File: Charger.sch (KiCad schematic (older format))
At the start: 2 parts

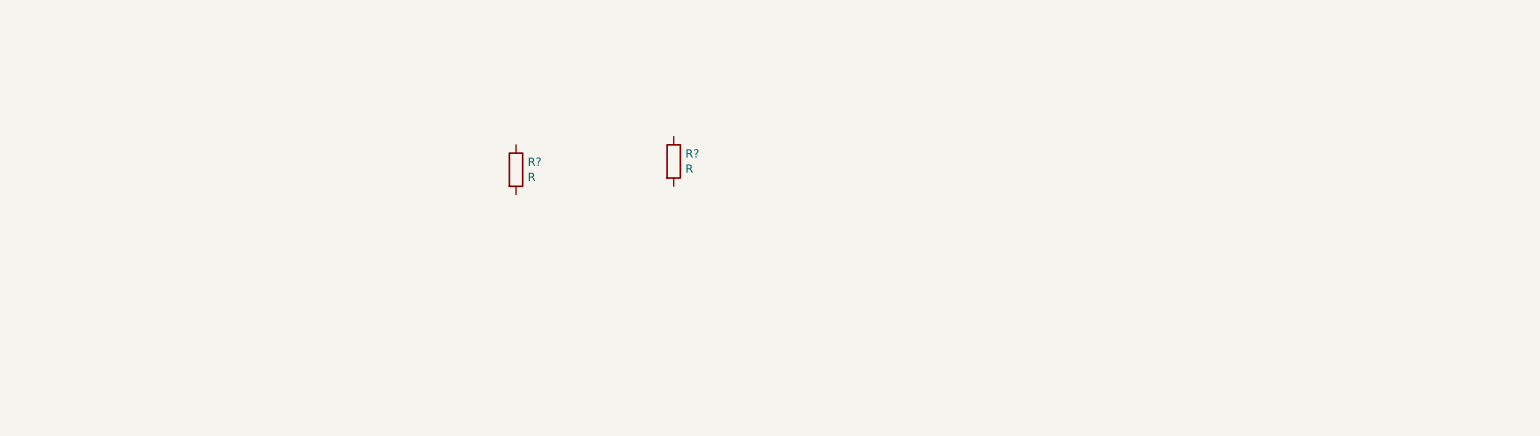
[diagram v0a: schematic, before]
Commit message: added ckt
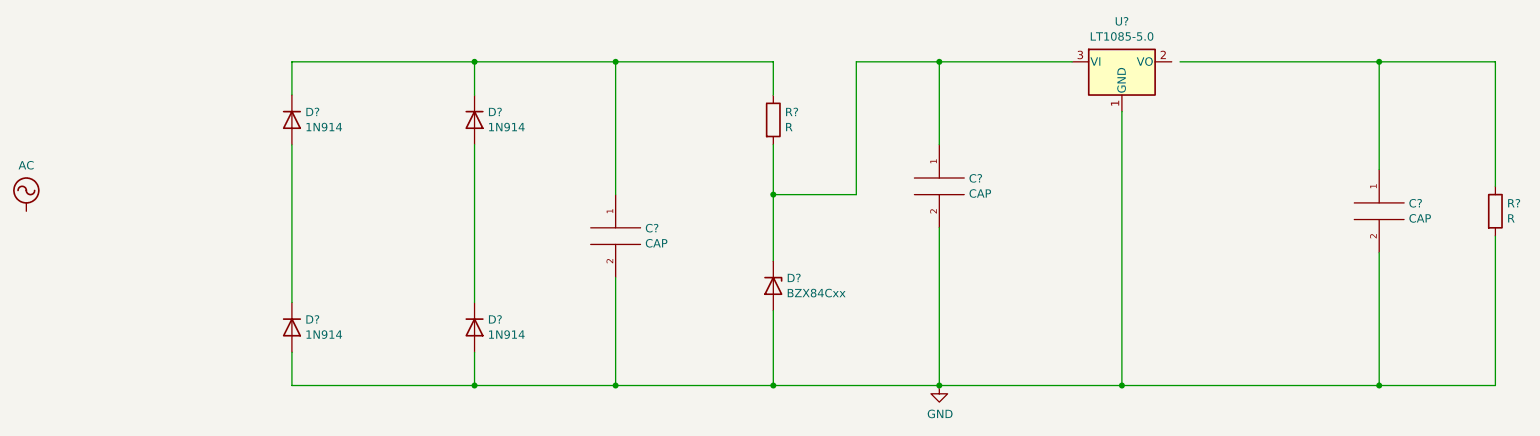
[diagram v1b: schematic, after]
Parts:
- removed R? (x2): R, symbol Device:R
- added C? (x3): CAP, symbol pspice:CAP
- added D? (x4): 1N914, Diode_THT:D_DO-35_SOD27_P7.62mm_Horizontal, symbol Diode:1N914
- added D?: BZX84Cxx, Diode_SMD:D_SOT-23_ANK, symbol Diode:BZX84Cxx
- added R? (x2): R, symbol Device:R
- added U?: LT1085-5.0, symbol Regulator_Linear:LT1085-5.0
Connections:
- net labels added: AC, GND
- wire segments 0 -> 35
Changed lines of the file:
@@
 $EndDescr
 $Comp
+L Diode:1N914 D?
+U 1 1 6031057C
+P 3100 2550
+F 0 "D?" V 3054 2630 50  0000 L CNN
+F 1 "1N914" V 3145 2630 50  0000 L CNN
+F 2 "Diode_THT:D_DO-35_SOD27_P7.62mm_Horizontal" H 3100 2375 50  0001 C CNN
+F 3 "http://www.vishay.com/docs/85622/1n914.pdf" H 3100 2550 50  0001 C CNN
+	1    3100 2550
+	0    1    1    0
+$EndComp
+$Comp
+L Diode:1N914 D?
+U 1 1 60311C82
+P 3100 3800
+F 0 "D?" V 3054 3880 50  0000 L CNN
+F 1 "1N914" V 3145 3880 50  0000 L CNN
+F 2 "Diode_THT:D_DO-35_SOD27_P7.62mm_Horizontal" H 3100 3625 50  0001 C CNN
+F 3 "http://www.vishay.com/docs/85622/1n914.pdf" H 3100 3800 50  0001 C CNN
+	1    3100 3800
+	0    1    1    0
+$EndComp
+$Comp
+L Diode:1N914 D?
+U 1 1 60312AAD
+P 4200 2550
+F 0 "D?" V 4154 2630 50  0000 L CNN
+F 1 "1N914" V 4245 2630 50  0000 L CNN
+F 2 "Diode_THT:D_DO-35_SOD27_P7.62mm_Horizontal" H 4200 2375 50  0001 C CNN
+F 3 "http://www.vishay.com/docs/85622/1n914.pdf" H 4200 2550 50  0001 C CNN
+	1    4200 2550
+	0    1    1    0
+$EndComp
+$Comp
+L Diode:1N914 D?
+U 1 1 60313CDB
+P 4200 3800
+F 0 "D?" V 4154 3880 50  0000 L CNN
+F 1 "1N914" V 4245 3880 50  0000 L CNN
+F 2 "Diode_THT:D_DO-35_SOD27_P7.62mm_Horizontal" H 4200 3625 50  0001 C CNN
+F 3 "http://www.vishay.com/docs/85622/1n914.pdf" H 4200 3800 50  0001 C CNN
+	1    4200 3800
+	0    1    1    0
+$EndComp
+$Comp
+L pspice:CAP C?
+U 1 1 60316869
+P 5050 3250
+F 0 "C?" H 5228 3296 50  0000 L CNN
+F 1 "CAP" H 5228 3205 50  0000 L CNN
+F 2 "" H 5050 3250 50  0001 C CNN
+F 3 "~" H 5050 3250 50  0001 C CNN
+	1    5050 3250
+	1    0    0    -1
+$EndComp
+$Comp
+L Diode:BZX84Cxx D?
+U 1 1 603170B0
+P 6000 3550
+F 0 "D?" V 5954 3630 50  0000 L CNN
+F 1 "BZX84Cxx" V 6045 3630 50  0000 L CNN
+F 2 "Diode_SMD:D_SOT-23_ANK" H 6000 3375 50  0001 C CNN
+F 3 "https://diotec.com/tl_files/diotec/files/pdf/datasheets/bzx84c2v4.pdf" H 6000 3550 50  0001 C CNN
+	1    6000 3550
+	0    1    1    0
+$EndComp
+$Comp
 L Device:R R?
-U 1 1 60309E92
-P 5400 2800
-F 0 "R?" H 5470 2846 50  0000 L CNN
-F 1 "R" H 5470 2755 50  0000 L CNN
-F 2 "" V 5330 2800 50  0001 C CNN
-F 3 "~" H 5400 2800 50  0001 C CNN
-	1    5400 2800
+U 1 1 60317AB7
+P 6000 2550
+F 0 "R?" H 6070 2596 50  0000 L CNN
+F 1 "R" H 6070 2505 50  0000 L CNN
+F 2 "" V 5930 2550 50  0001 C CNN
+F 3 "~" H 6000 2550 50  0001 C CNN
+	1    6000 2550
+	1    0    0    -1
+$EndComp
+$Comp
+L pspice:CAP C?
+U 1 1 60318512
+P 7000 2950
+F 0 "C?" H 7178 2996 50  0000 L CNN
+F 1 "CAP" H 7178 2905 50  0000 L CNN
+F 2 "" H 7000 2950 50  0001 C CNN
+F 3 "~" H 7000 2950 50  0001 C CNN
+	1    7000 2950
+	1    0    0    -1
+$EndComp
+$Comp
+L pspice:CAP C?
+U 1 1 6031AA99
+P 9650 3100
+F 0 "C?" H 9828 3146 50  0000 L CNN
+F 1 "CAP" H 9828 3055 50  0000 L CNN
+F 2 "" H 9650 3100 50  0001 C CNN
+F 3 "~" H 9650 3100 50  0001 C CNN
+	1    9650 3100
 	1    0    0    -1
 $EndComp
 $Comp
 L Device:R R?
-U 1 1 6030A5AE
-P 4450 2850
-F 0 "R?" H 4520 2896 50  0000 L CNN
-F 1 "R" H 4520 2805 50  0000 L CNN
-F 2 "" V 4380 2850 50  0001 C CNN
-F 3 "~" H 4450 2850 50  0001 C CNN
-	1    4450 2850
-	1    0    0    -1
-$EndComp
+U 1 1 6031AFD1
+P 10350 3100
+F 0 "R?" H 10420 3146 50  0000 L CNN
+F 1 "R" H 10420 3055 50  0000 L CNN
+F 2 "" V 10280 3100 50  0001 C CNN
+F 3 "~" H 10350 3100 50  0001 C CNN
+	1    10350 3100
+	1    0    0    -1
+$EndComp
+$Comp
+L Regulator_Linear:LT1085-5.0 U?
+U 1 1 6031B799
+P 8100 2200
+F 0 "U?" H 8100 2442 50  0000 C CNN
+F 1 "LT1085-5.0" H 8100 2351 50  0000 C CNN
+F 2 "" H 8100 2450 50  0001 C CIN
+F 3 "https://www.analog.com/media/en/technical-documentation/data-sheets/1083ffe.pdf" H 8100 2200 50  0001 C CNN
+	1    8100 2200
+	1    0    0    -1
+$EndComp
+Wire Wire Line
+	8450 2200 9650 2200
+Wire Wire Line
+	3100 3950 3100 4150
+Wire Wire Line
+	3100 4150 4200 4150
+Wire Wire Line
+	4200 4150 4200 3950
+Wire Wire Line
+	4200 3650 4200 2700
+Wire Wire Line
+	4200 2400 4200 2200
+Wire Wire Line
+	4200 2200 3100 2200
+Wire Wire Line
+	3100 2200 3100 2400
+Wire Wire Line
+	3100 2700 3100 3650
+Wire Wire Line
+	5050 3000 5050 2200
+Wire Wire Line
+	5050 2200 4200 2200
+Connection ~ 4200 2200
+Wire Wire Line
+	5050 3500 5050 4150
+Wire Wire Line
+	5050 4150 4200 4150
+Connection ~ 4200 4150
+Wire Wire Line
+	6000 4150 6000 3700
+Wire Wire Line
+	6000 3400 6000 3000
+Wire Wire Line
+	6000 2400 6000 2200
+Wire Wire Line
+	6000 2200 5050 2200
+Connection ~ 5050 2200
+Wire Wire Line
+	6000 3000 6500 3000
+Wire Wire Line
+	6500 3000 6500 2200
+Wire Wire Line
+	6500 2200 7000 2200
+Wire Wire Line
+	7000 2200 7000 2700
+Connection ~ 6000 3000
+Wire Wire Line
+	6000 3000 6000 2700
+Wire Wire Line
+	7000 3200 7000 4150
+Wire Wire Line
+	7000 4150 6000 4150
+Connection ~ 6000 4150
+Wire Wire Line
+	5050 4150 6000 4150
+Connection ~ 5050 4150
+Wire Wire Line
+	7000 2200 7800 2200
+Connection ~ 7000 2200
+Wire Wire Line
+	7000 4150 8100 4150
+Wire Wire Line
+	10350 4150 10350 3250
+Connection ~ 7000 4150
+Connection ~ 9650 4150
+Wire Wire Line
+	9650 4150 10350 4150
+Connection ~ 9650 2200
+Wire Wire Line
+	9650 2200 10350 2200
+Wire Wire Line
+	9650 3350 9650 4150
+Wire Wire Line
+	9650 2200 9650 2850
+Wire Wire Line
+	10350 2200 10350 2950
+Wire Wire Line
+	8100 2500 8100 4150
+Connection ~ 8100 4150
+Wire Wire Line
+	8100 4150 9650 4150
+$Comp
+L power:GND #PWR?
+U 1 1 6032C60B
+P 7000 4150
+F 0 "#PWR?" H 7000 3900 50  0001 C CNN
+F 1 "GND" H 7005 3977 50  0000 C CNN
+F 2 "" H 7000 4150 50  0001 C CNN
+F 3 "" H 7000 4150 50  0001 C CNN
+	1    7000 4150
+	1    0    0    -1
+$EndComp
+$Comp
+L power:AC #PWR?
+U 1 1 6032CF48
+P 1500 3100
+F 0 "#PWR?" H 1500 3000 50  0001 C CNN
+F 1 "AC" H 1500 3375 50  0000 C CNN
+F 2 "" H 1500 3100 50  0001 C CNN
+F 3 "" H 1500 3100 50  0001 C CNN
+	1    1500 3100
+	1    0    0    -1
+$EndComp
